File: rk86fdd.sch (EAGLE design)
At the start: 23 parts

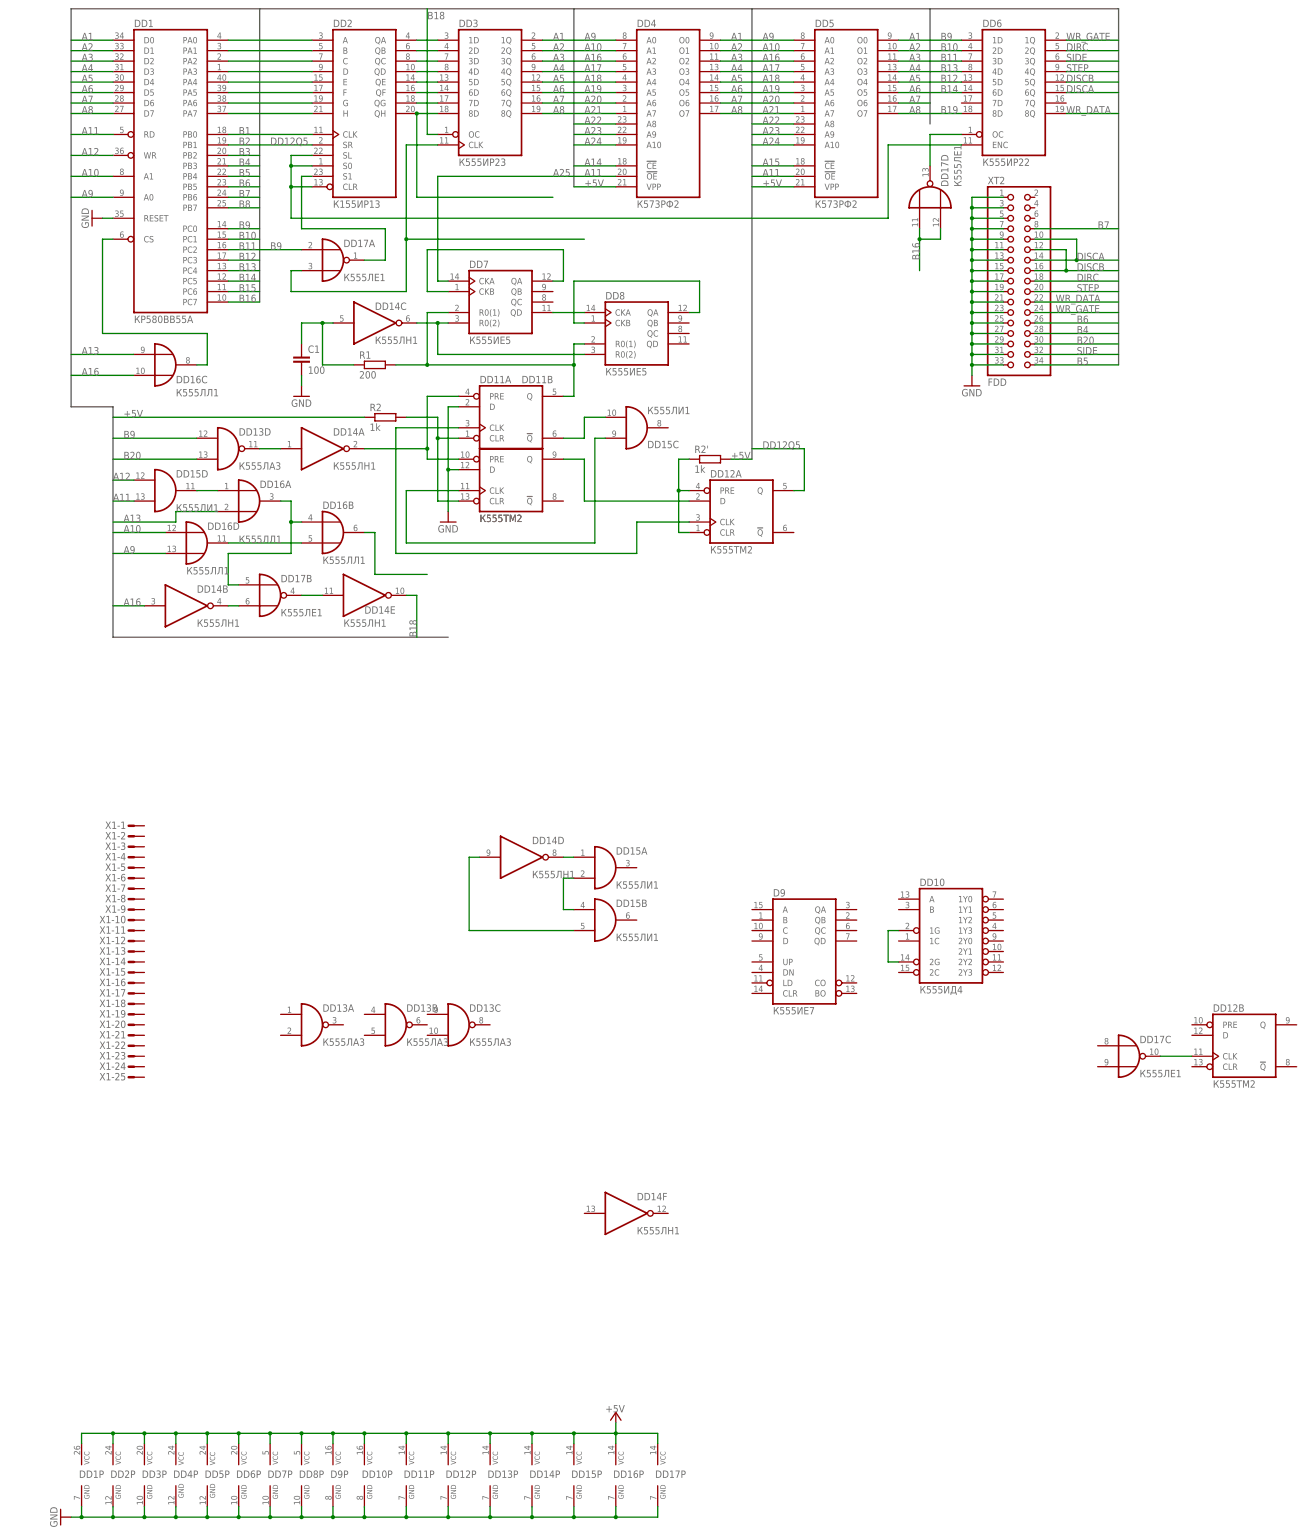
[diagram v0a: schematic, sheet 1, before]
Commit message: .
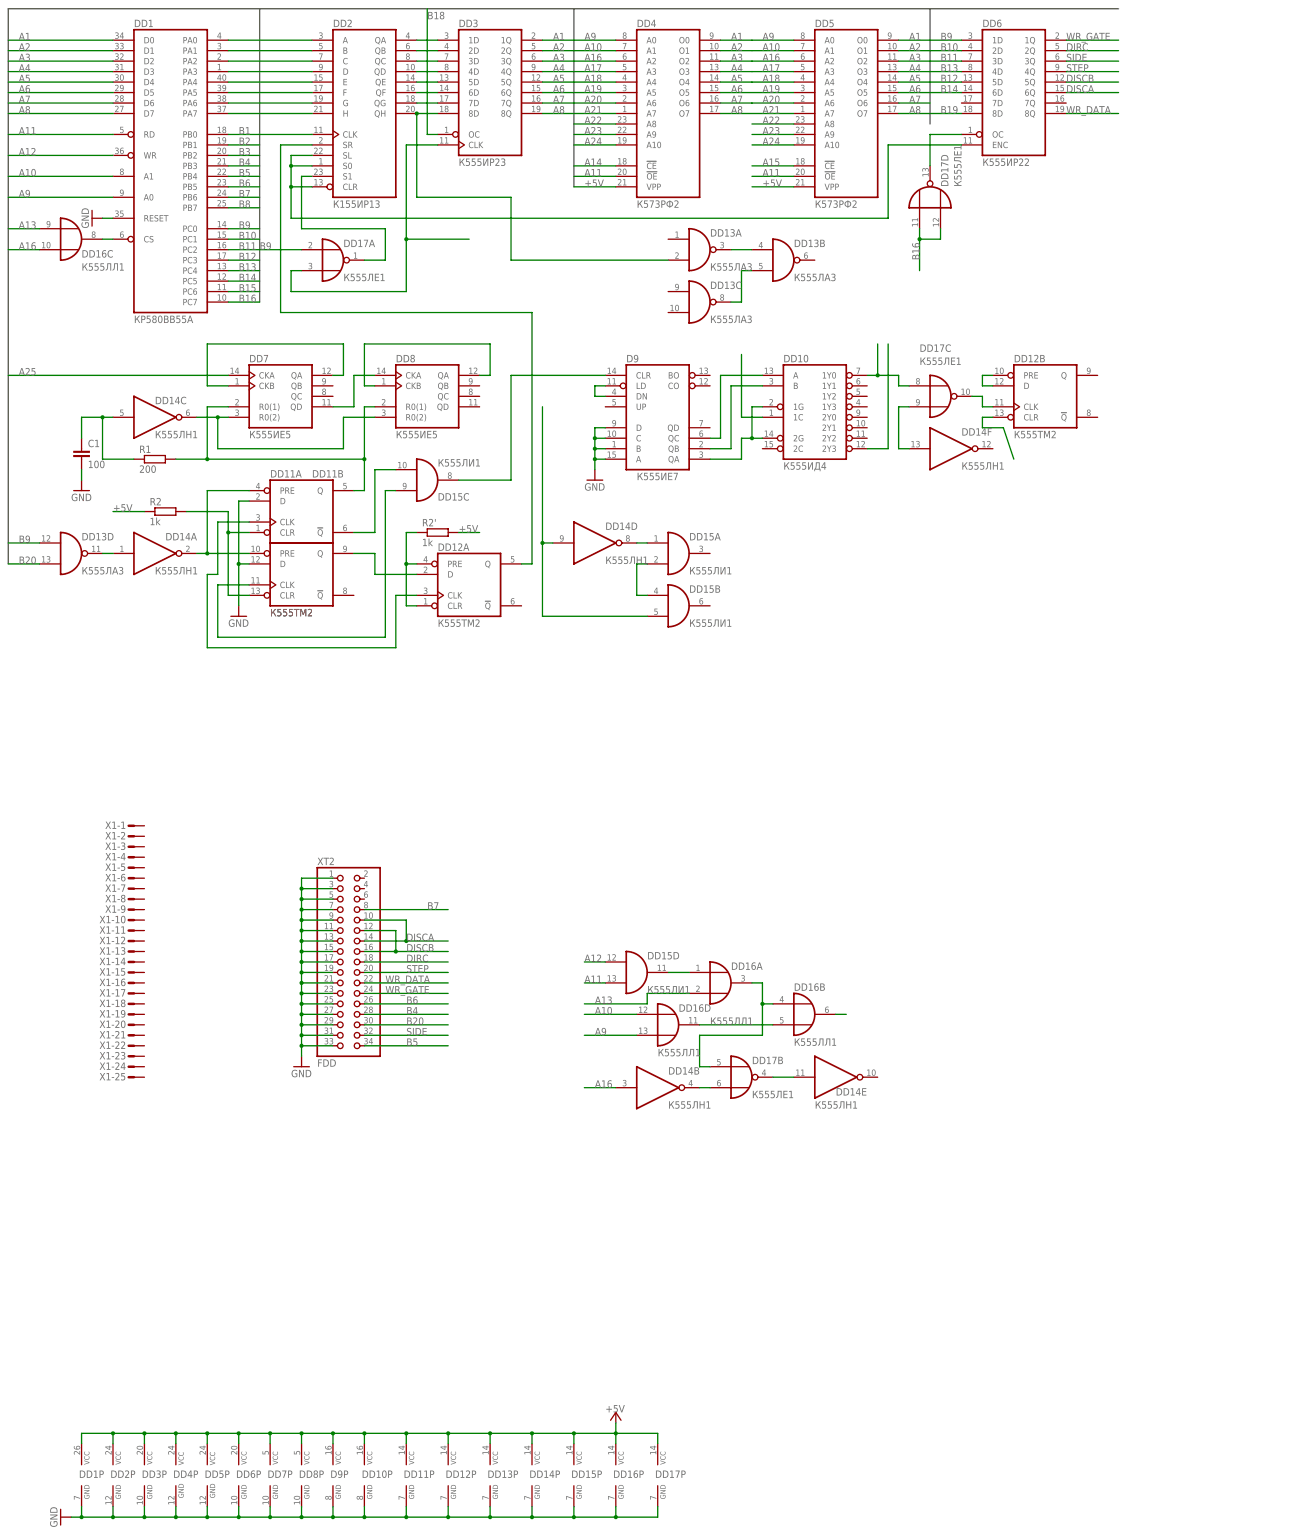
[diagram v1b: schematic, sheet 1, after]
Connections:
- new net N$33: DD10A.1C
- new net N$45: DD13A.O, DD13B.I0
- new net N$46: DD13B.I1, DD13C.O
- new net N$48: D9A.CLR, DD15C.O
- new net N$49: D9A.QB, DD10A.B
- new net N$50: D9A.QC, DD10A.A
- new net N$52: D9A.DN, D9A.LD
- new net N$53: DD14F.I, DD17C.I1
- new net N$54: DD12B.CLR
- new net N$55: DD12B.D, DD12B.PRE
- new net N$56: DD10A.1Y0, DD17C.I0
- new net N$57: DD10A.2Y3
- net B18: no longer DD14E.O
- net GND: now also D9A.A, D9A.B, D9A.C, D9A.D
- net N$34: now also D9A.QA
- net N$9: now also DD13A.I1
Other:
- moved on the sheet: C1, D9, DD10, DD11A, DD11B, DD12A, DD12B, DD13A, DD13B, DD13C, DD13D, DD14A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
